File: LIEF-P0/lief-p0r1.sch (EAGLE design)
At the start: 14 parts, among them U1 MPL3115A2LGA8, U2 L3G4200D, U3 HMC6343A

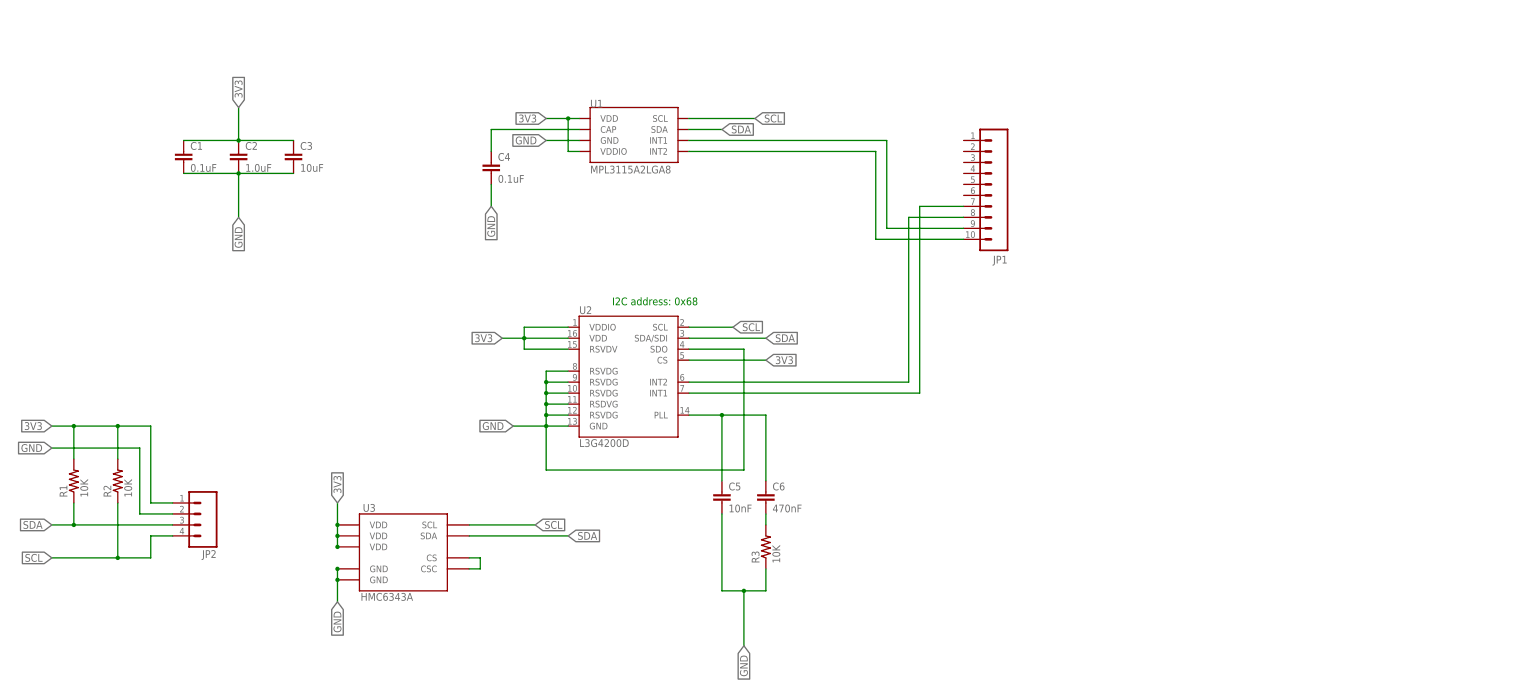
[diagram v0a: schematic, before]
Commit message: Revision 3 of the LIEF hardware design.
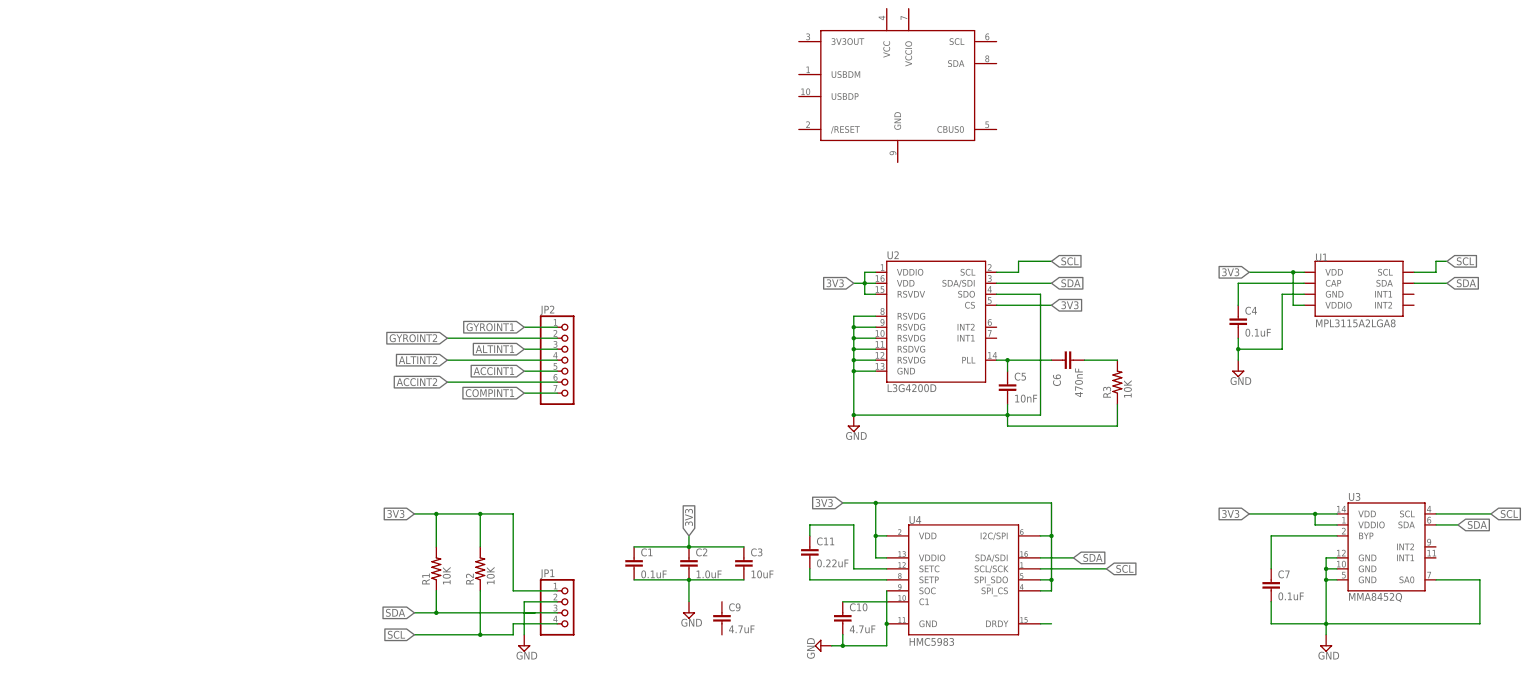
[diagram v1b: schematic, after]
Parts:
- added C10: 4.7uF, SparkFun-Capacitors:1.0UF-25V-+80/-20(0805)"
- added C11: 0.22uF, SparkFun-Capacitors:1.0UF-25V-+80/-20(0805)"
- added C7: 0.1uF, SparkFun-Capacitors:0.1UF-100V-10%(0603)
- added C9: 4.7uF, SparkFun-Capacitors:0.1UF-100V-10%(0603)
- added U$1: FT200XD, Synapseware:FT200XD
- added U4: (no value), bitfab:HMC5983
- JP1: device SparkFun-Connectors:M10LOCK -> pinhead:PINHD-1X4
- JP2: device SparkFun-Connectors:M04LOCK -> pinhead:PINHD-1X7
- U3: value HMC6343A -> MMA8452Q; device SparkFun-Sensors:HMC6343A -> SparkFun-Sensors:MMA8452Q
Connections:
- removed net N$1: JP1.10, U1.INT2
- removed net N$2: U3.CS, U3.CSC
- removed net N$3: JP1.9, U1.INT1
- removed net N$4: JP1.7, U2.INT1
- new net ACCINT1: JP2.5
- new net ACCINT2: JP2.6
- new net ALTINT1: JP2.3
- new net ALTINT2: JP2.4
- new net COMPINT1: JP2.7
- new net GYROINT1: JP2.1
- new net GYROINT2: JP2.2
- new net N$10: C11.2, U4.SETP
- new net N$12: C10.1, U4.C1
- new net N$19: U4.DRDY
- new net N$9: C7.1, U3.BYP
- net 3V3: now also JP1.1, U3.VDD, U3.VDDIO, U4.I2C/SPI, U4.SPI_CS, U4.SPI_SDO, U4.VDD, U4.VDDIO; no longer JP2.1, U3.VDD@11, U3.VDD@21, U3.VDD@3
- net GND: now also C10.2, C7.2, JP1.2, JP1.3, U3.GND@0, U3.GND@1, U3.GND@2, U3.SA0, U4.GND, U4.SOC; no longer JP2.2, U3.GND@25, U3.GND@29
- net N$5: now also C11.1, U4.SETC; no longer JP1.8, U2.INT2
- net SCL: now also JP1.4, U4.SCL/SCK; no longer JP2.4
- net SDA: now also U4.SDA/SDI; no longer JP2.3
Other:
- note added: "1 mA"
- note added: "2 mA"
- note added: "7 mA"
- note added: "Accelerometer"
- note added: "Altimeter & Thermometer"
- note added: "Board-to-Board Interface Header"
- note added: "Compass"
- note added: "FT200XD"
- note added: "Gyroscope"
- note added: "I2C address: 0x1D (7bit)"
- note added: "I2C address: 0x1E (7bit)"
- note added: "I2C address: 0x60 (7bit) 0xC1 (8bit read) 0xC0 (8bit write)"
- note added: "I2C address: 0x68 (7bit)"
- note added: "Power Filter"
- note added: "Todo ==== * connect the FTDI FT200XD * reduce power filter (see arduino schem) * add CBUS (ethernet) connector * check packages of all parts * enhance FT200XD symbol * coalesce all parts into bitfab.lbr"
- note removed: "I2C address: 0x68"
- moved on the sheet: C1, C2, C3, C4, C5, C6, R1, R2, R3, U1, U2
